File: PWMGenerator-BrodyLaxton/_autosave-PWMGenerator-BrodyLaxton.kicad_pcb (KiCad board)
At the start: 2 copper layers, 176.8 x 118.4 mm, 30 parts, among them J1 Conn_01x03_Pin, Q1 2N3904, Q2 2N3904, Q3 2N3906, Q4 2N3906, SW2 SW_SPST, U1 LM339, U2 LM7805_TO220

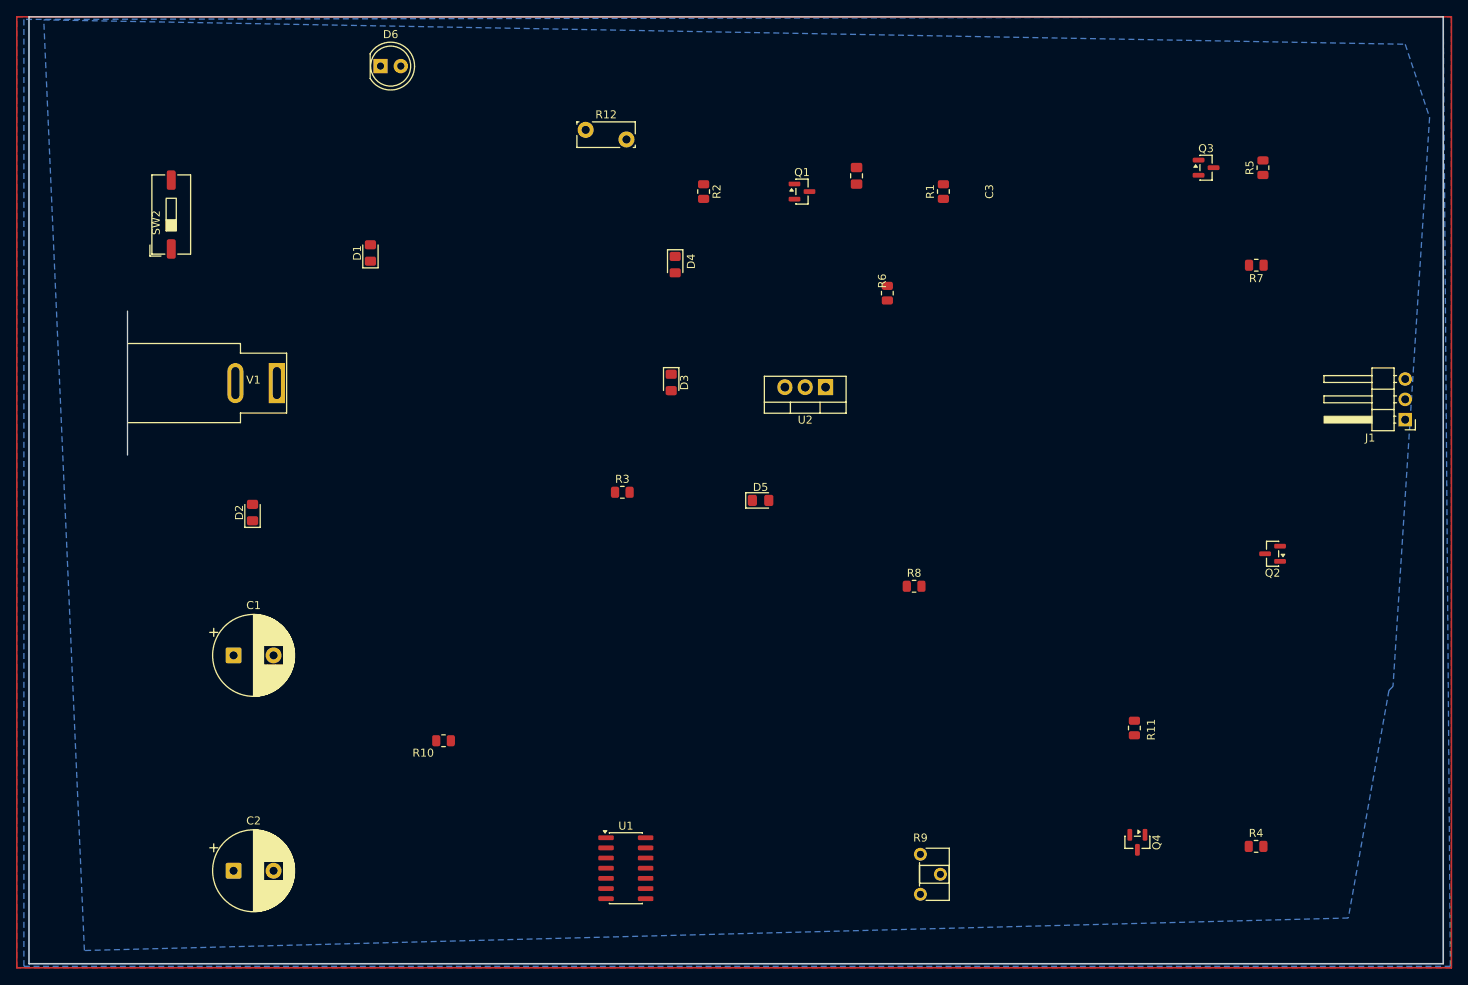
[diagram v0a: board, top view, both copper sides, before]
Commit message: PART 2 REDONE
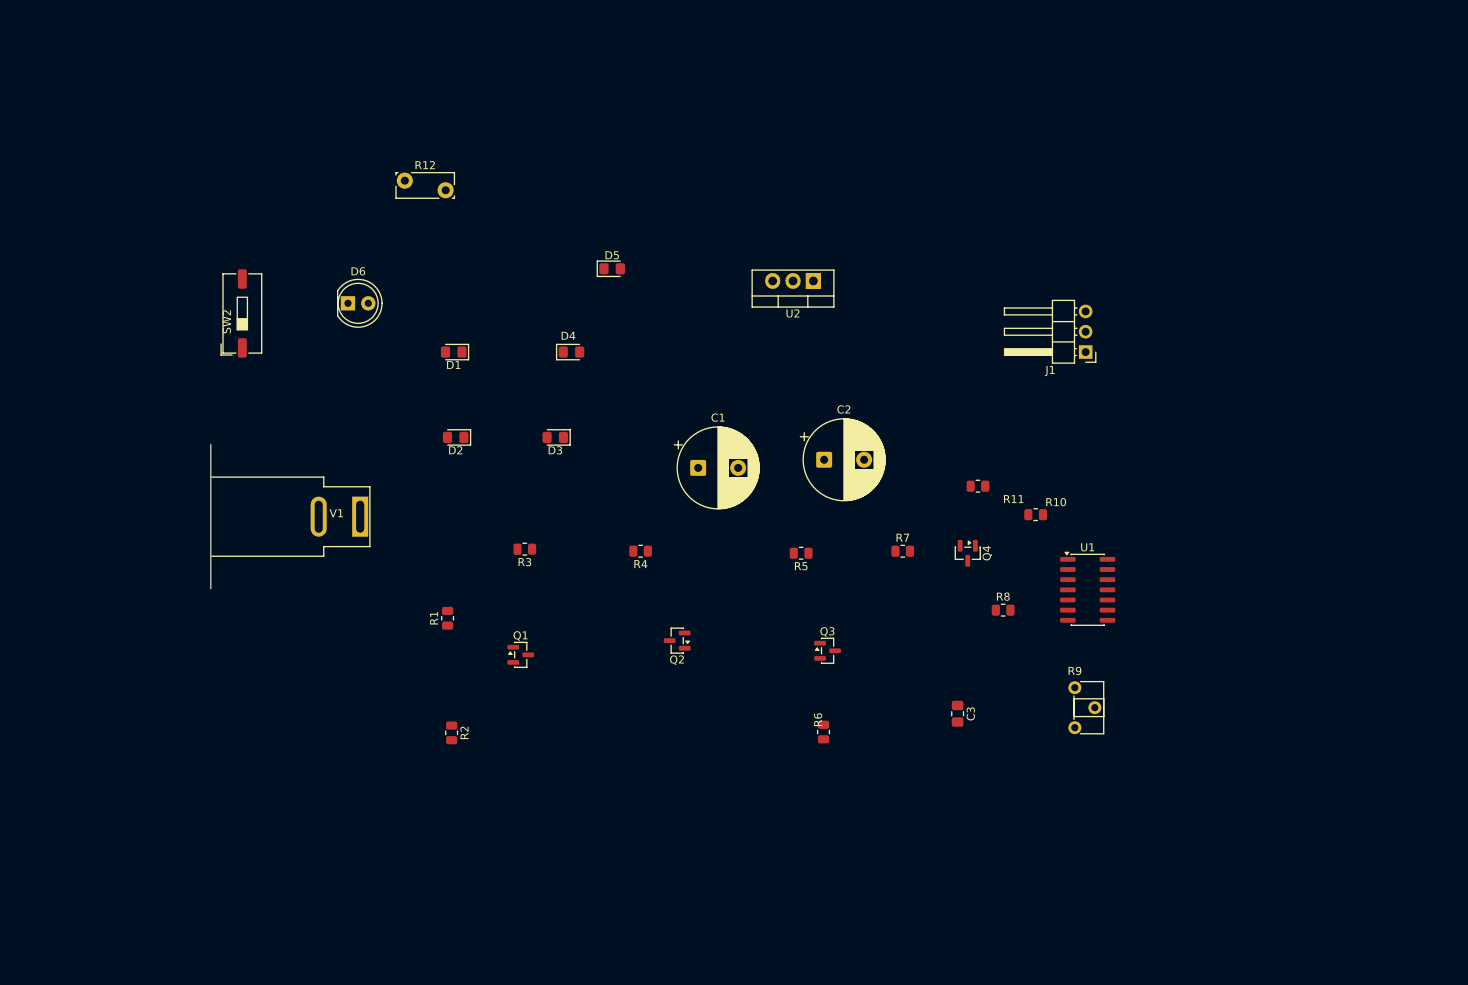
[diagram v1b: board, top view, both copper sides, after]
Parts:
- moved C2 89.9 mm to (151.7, 85.3)
- moved R4 85.3 mm to (128.8, 96.8), turned to 180 degrees
- moved R1 81.8 mm to (104.6, 105.2)
- moved R10 79.2 mm to (178.2, 92.2), turned to 180 degrees
- moved Q3 76.7 mm to (152.1, 109.2)
- moved Q2 75.2 mm to (133.3, 108.0)
- moved R5 75.2 mm to (148.8, 97.0), turned to 180 degrees
- moved R2 74.6 mm to (105.2, 119.5)
- moved C3 68.4 mm to (168.4, 117.1), turned to -90 degrees
- moved Q1 67.7 mm to (113.8, 109.7)
- moved U1 67.4 mm to (184.7, 101.6)
- moved C1 62.6 mm to (136.0, 86.4)
- moved R7 56.8 mm to (161.5, 96.8), turned to 0 degrees
- moved R6 55.4 mm to (151.6, 119.4)
- moved Q4 41.9 mm to (169.7, 97.0)
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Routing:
- removed copper zone on B.Cu, net GNDREF
- removed copper zone on F.Cu, net VCC
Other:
- board outline removed
